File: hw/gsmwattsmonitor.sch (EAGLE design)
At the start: 9 parts

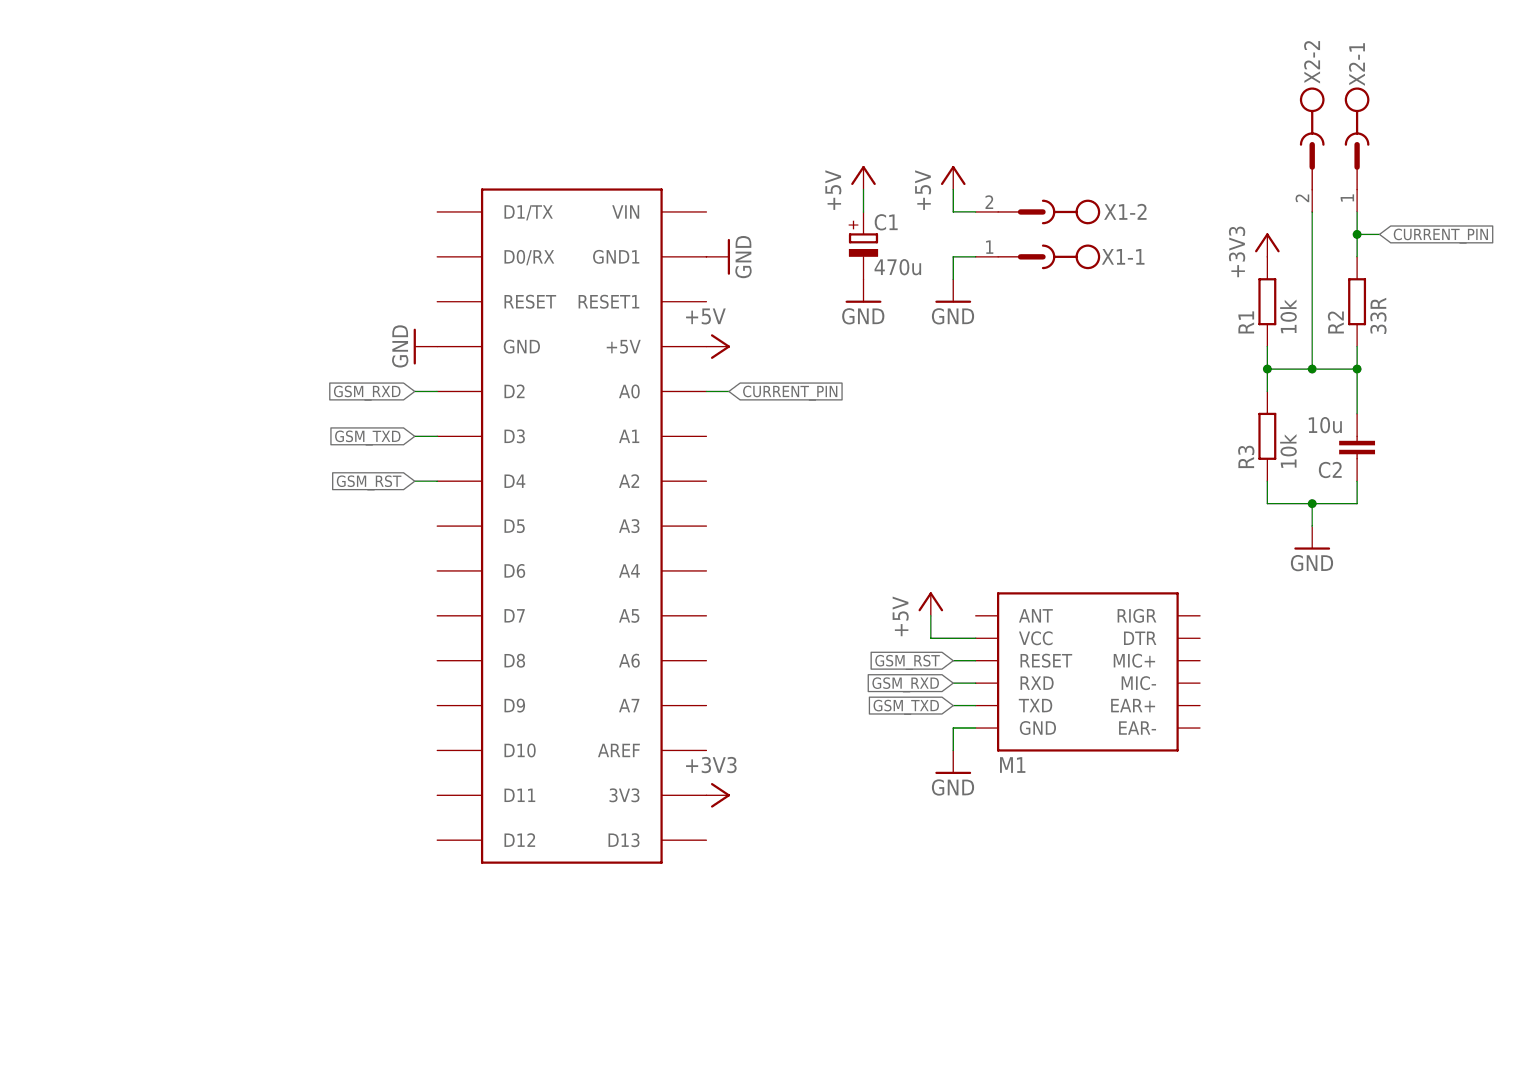
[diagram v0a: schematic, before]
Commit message: updated hardware
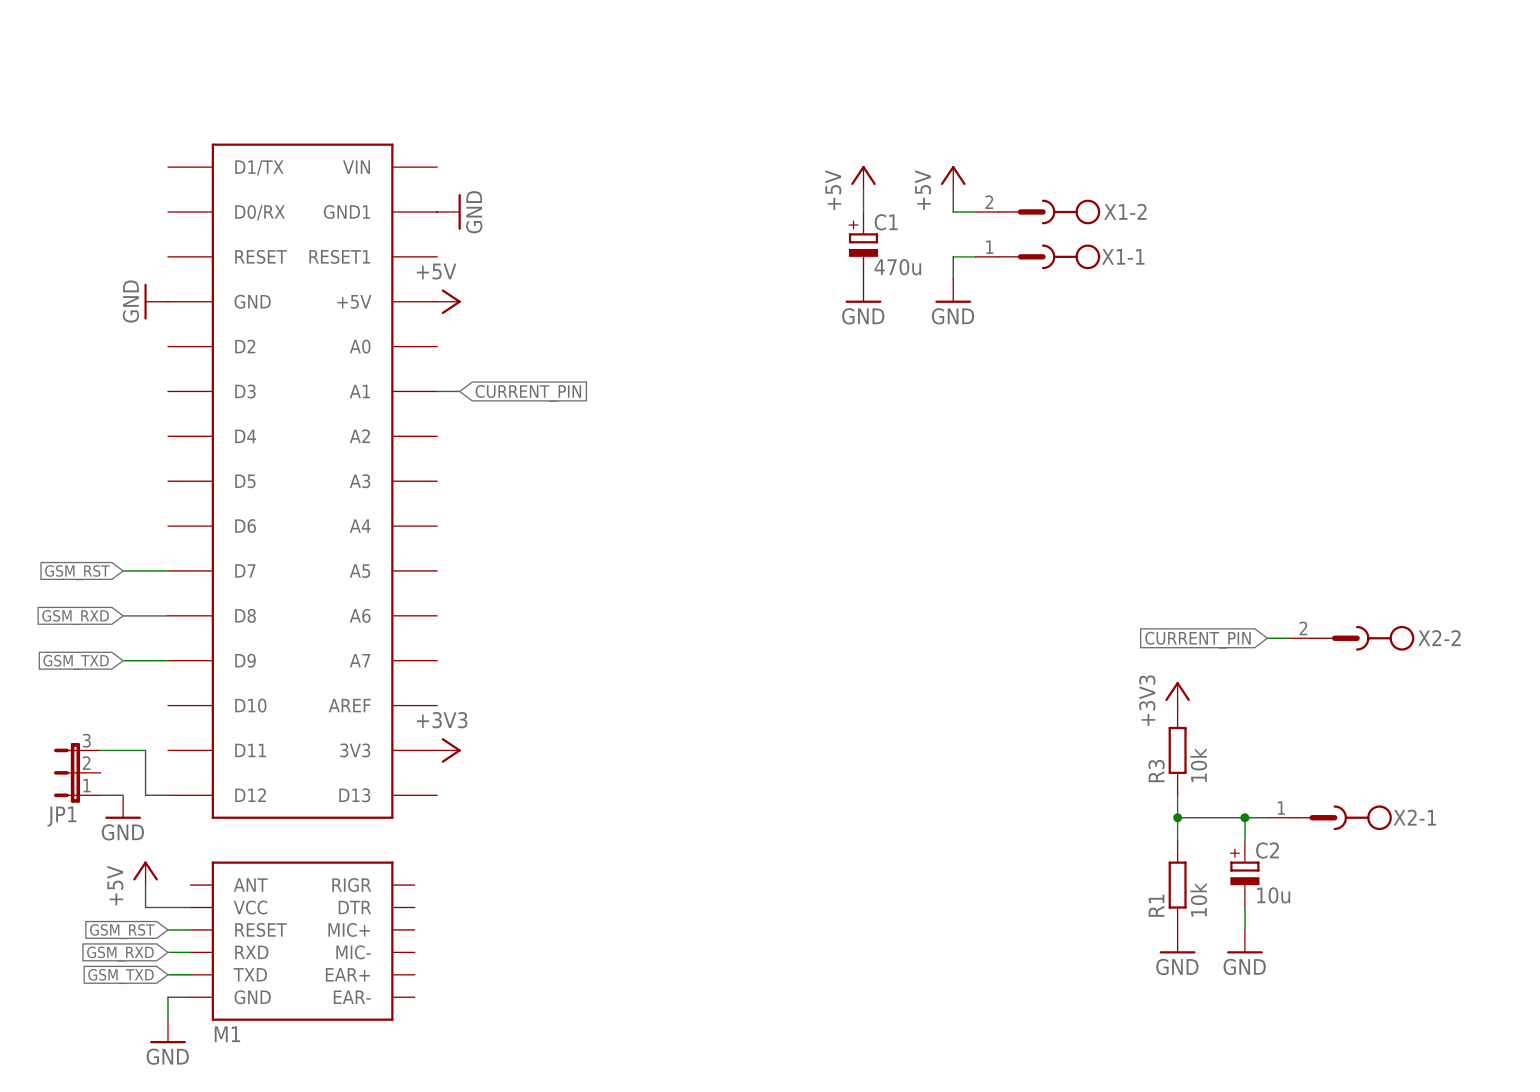
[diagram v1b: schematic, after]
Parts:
- removed R2: 33R, rcl:R-EU_R0805
- added JP1: (no value), jumper:JP2E
- C1: device rcl:CPOL-EUSANYO_SMD_E7 -> rcl:CPOL-EUE2.5-6
- C2: device rcl:C-EUC0805 -> rcl:CPOL-EUE2-4
- R1, R3: device rcl:R-EU_R0805 -> rcl:R-EU_0204/7
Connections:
- new net N$2: JP1.3, U$1.D12
- net +3V3: now also R3.2; no longer R1.2
- net CURRENT_PIN: now also U$1.A1, X2-2.SK; no longer R2.2, U$1.A0, X2-1.SK
- net GND: now also C2.-, JP1.1, R1.1; no longer C2.1, R3.1
- net GSM_RST: now also U$1.D7; no longer U$1.D4
- net GSM_RXD: now also U$1.D8; no longer U$1.D2
- net GSM_TXD: now also U$1.D9; no longer U$1.D3
- net N$1: now also C2.+, R1.2, R3.1, X2-1.SK; no longer C2.2, R1.1, R2.1, R3.2, X2-2.SK
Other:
- moved on the sheet: M1, R1, R3, X2-1, X2-2
